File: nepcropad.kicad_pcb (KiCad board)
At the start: 2 copper layers, 99.2 x 58.7 mm, 34 parts, among them SW1 SW_Push, U1 ATmega32U4-A, Y1 16MHz

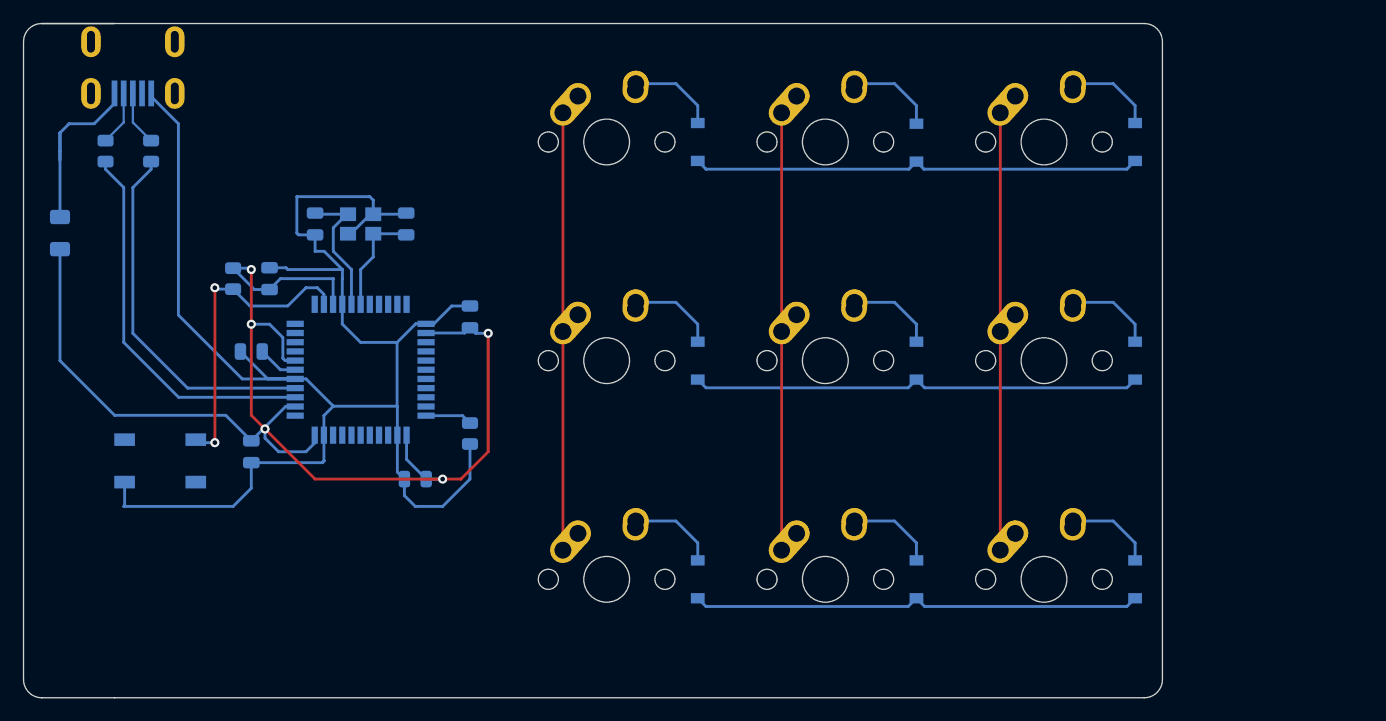
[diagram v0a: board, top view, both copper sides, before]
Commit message: Finished routing
I think atleast.
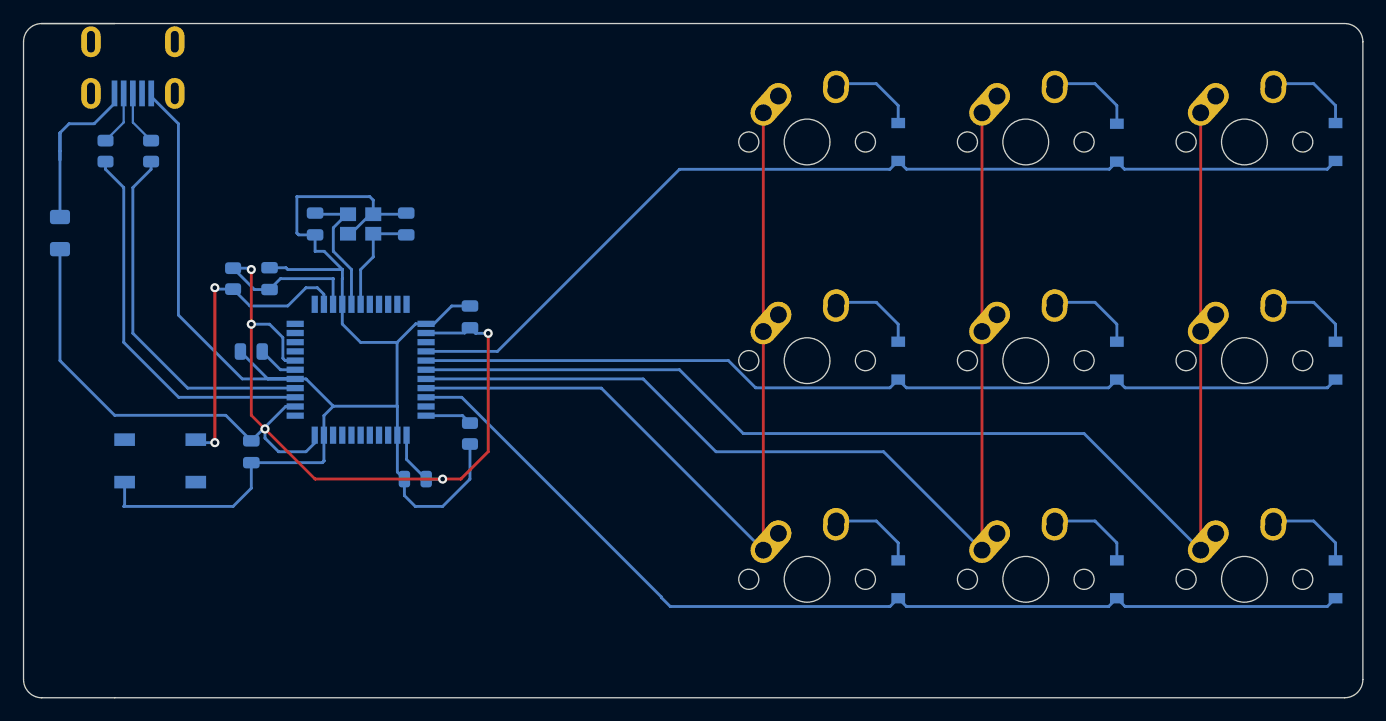
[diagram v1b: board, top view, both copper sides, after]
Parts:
- moved D1 17.5 mm to (158.0, 71.4)
- moved D2 17.5 mm to (177.0, 71.5)
- moved D3 17.5 mm to (196.1, 71.4)
- moved D4 17.5 mm to (158.0, 90.5)
- moved D5 17.5 mm to (177.0, 90.5)
- moved D6 17.5 mm to (196.1, 90.5)
- moved D7 17.5 mm to (158.0, 109.5)
- moved D8 17.5 mm to (177.0, 109.5)
- moved D9 17.5 mm to (196.1, 109.5)
- moved MX1 17.5 mm to (150.0, 71.4)
- moved MX2 17.5 mm to (169.1, 71.4)
- moved MX3 17.5 mm to (188.1, 71.4)
- moved MX4 17.5 mm to (150.0, 90.5)
- moved MX5 17.5 mm to (169.1, 90.5)
- moved MX6 17.5 mm to (188.1, 90.5)
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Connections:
- U1 pad 26: unconnected-(U1-Pad26) -> ROW0
- U1 pad 27: unconnected-(U1-Pad27) -> ROW1
- U1 pad 28: unconnected-(U1-Pad28) -> COL2
- U1 pad 29: unconnected-(U1-Pad29) -> COL1
- U1 pad 30: unconnected-(U1-Pad30) -> COL0
- U1 pad 31: unconnected-(U1-Pad31) -> ROW2
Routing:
- net COL2: track 38.1 -> 112.1 mm
- net COL1: track 38.1 -> 92.7 mm
- net ROW2: track 39.3 -> 88.3 mm
- net ROW0: track 39.2 -> 87.2 mm
- net ROW1: track 39.3 -> 81.7 mm
- net COL0: track 38.1 -> 73.3 mm
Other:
- board size 99.2 x 58.7 mm -> 116.7 x 58.7 mm
